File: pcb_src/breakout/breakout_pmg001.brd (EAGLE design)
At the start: 25.4 x 60.3 mm, 26 parts

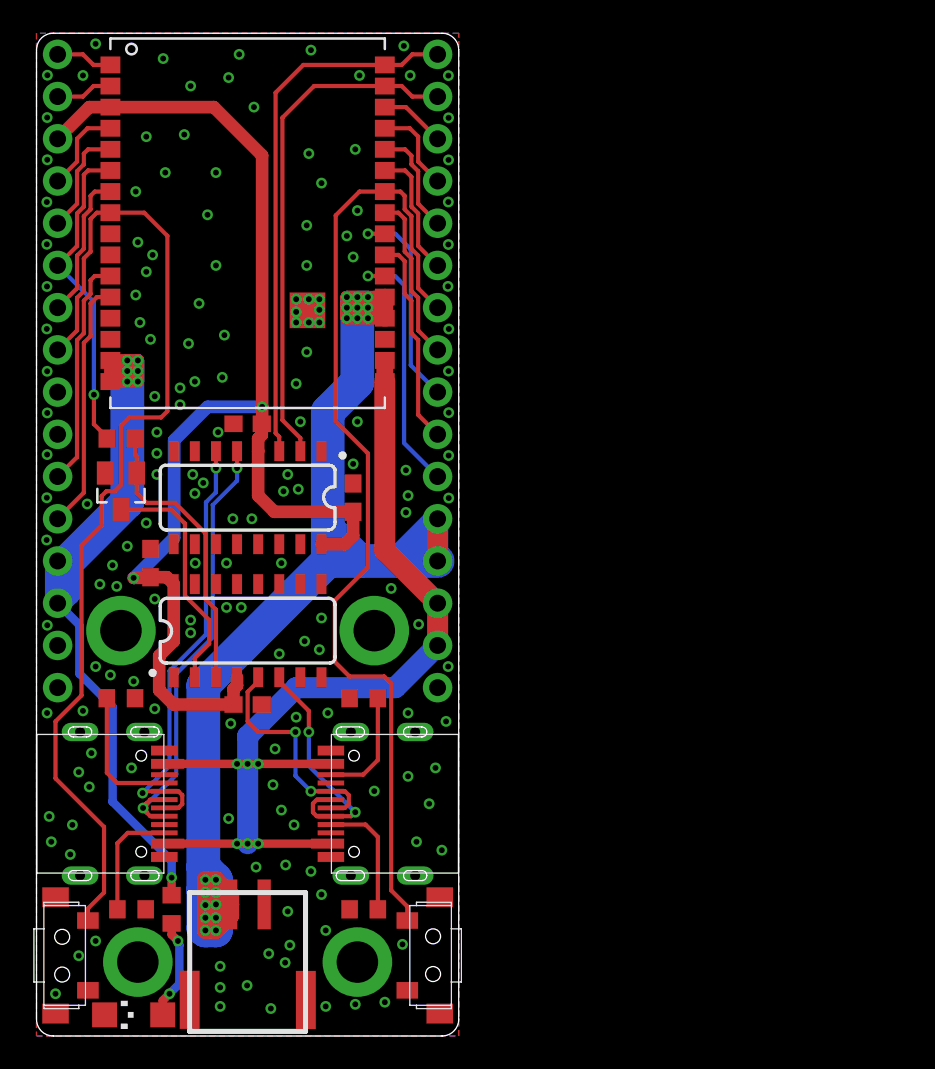
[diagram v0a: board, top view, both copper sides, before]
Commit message: Reworked repository
Name changed, added a lot of new resources etc.
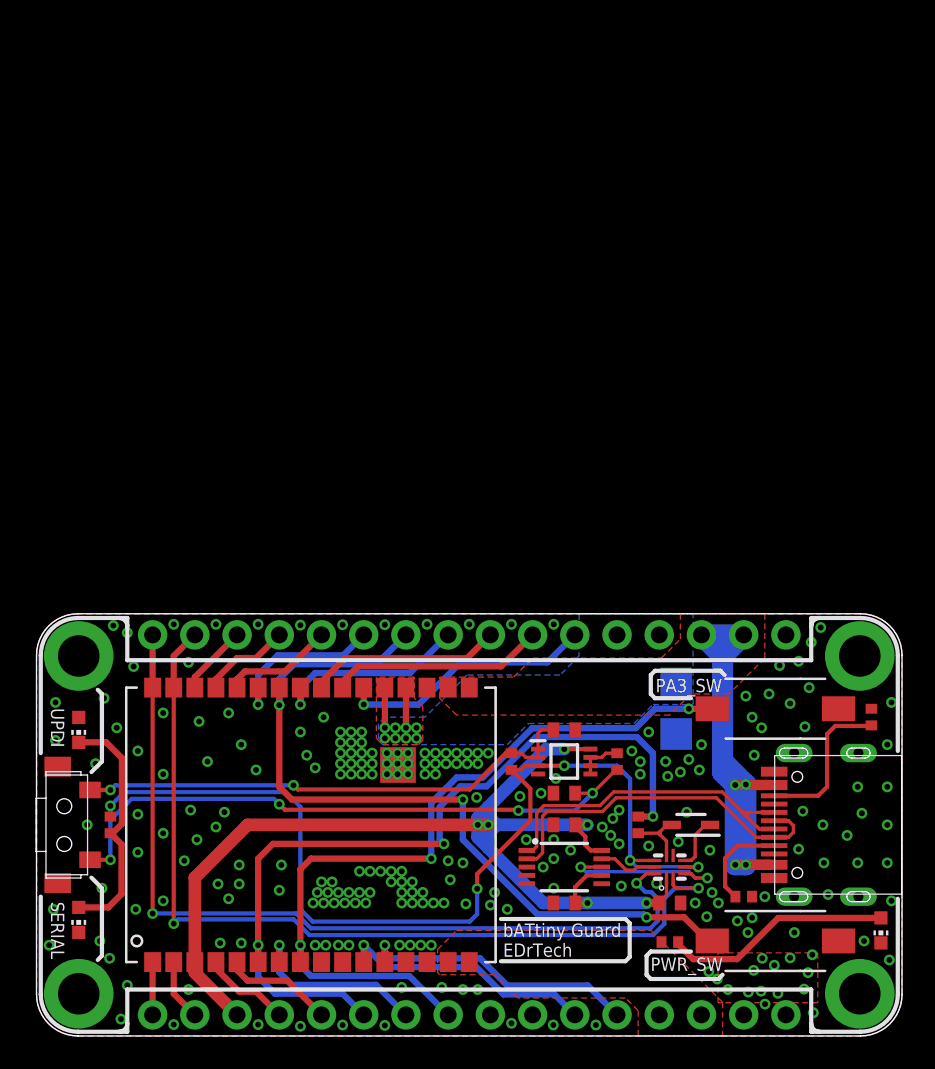
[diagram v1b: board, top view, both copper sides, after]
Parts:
- removed C3, C4, C5, C6: 100nF, eagle-ltspice:C0603
- removed LED1: (no value), led:CHIPLED_1206
- removed R11, R12, R7: 5.1k, rcl:R0603
- removed R8: 470R, rcl:R0603
- removed SPEAKER_CON1: JST_HEADER_2MM_2P, edrtech_lib:JST_HEADER
- removed U$3: TS-1101VS-C-A-A, circuitmess_device_library:TS-1101VS-C-A-A
- removed U$5: CH340C, circuitmess_device_library:CH340C
- removed U$6: USB-C, edrtech_lib:USB-C
- added C1: 1u, rcl:C0402
- added C2: 10n, rcl:C0402
- added C7, C8, C9: 100nF, rcl:C0402
- added IC1: SN74AUP2G00DCUR, SN74AUP2G00DCUR:SOP50P310X90-8N
- added LED2, LED4, LED5: (no value), led:CHIP-LED0603
- added R1: 100k, rcl:R0402
- added R2: 10k, rcl:R0402
- added R3, R4: 5.1k, rcl:R0402
- added R9: 470R, rcl:R0402
- added S5: TS3A5223RSWR, TS3A5223RSWR:RSW(RPUQFNN10)
- added TP1, TP2: TPSQTP19SQ, testpad:TP19SQ
- added U$12: USB-C, edrtech_lib:USB-C
- added U2: CH340E_MSOP10, CH340E:MSOP10
- D1: value BAT54 -> BAT54WS-13P; device diode:SOT23 -> BAT54WS-13P:SOD2512X115N
- R5, R6: device rcl:R0603 -> rcl:R0402
- U$1: value CH340C -> TS-1101S; device circuitmess_device_library:CH340C -> edrtech_lib:TS-1101S
- U$4: value USB-C -> TS-1101S; device edrtech_lib:USB-C -> edrtech_lib:TS-1101S
- moved U$9 47.2 mm to (49.5, 22.9), turned to 90 degrees
- moved JP1 46.0 mm to (26.0, 1.27), turned to 0 degrees
- moved U$4 41.5 mm to (44.5, 5.71), turned to 180 degrees
- moved D1 39.7 mm to (39.4, 12.7)
- moved U$7 36.4 mm to (16.5, 12.7), turned to 90 degrees
- moved U$1 34.2 mm to (44.5, 19.7)
- moved U$8 30.3 mm to (49.5, 2.54), turned to 90 degrees
- moved R5 30.0 mm to (38.1, 5.65), turned to 180 degrees
- moved U$10 22.0 mm to (2.54, 2.54), turned to 90 degrees
- moved U$11 17.8 mm to (2.54, 22.9), turned to 90 degrees
- moved R6 16.1 mm to (4.45, 12.7), turned to 90 degrees
- moved JP2 16.0 mm to (26.0, 24.1), turned to 180 degrees
- moved U$2 7.86 mm to (1.27, 12.7)
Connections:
- removed net D+_AT: U$1.5, U$4.DP1, U$4.DP2
- removed net D+_U: U$5.5, U$6.DP1, U$6.DP2
- removed net D-_AT: U$1.6, U$4.DN1, U$4.DN2
- removed net D-_U: U$5.6, U$6.DN1, U$6.DN2
- removed net N$5: R7.1, U$6.CC2
- removed net N$8: R11.2, U$4.CC1
- removed net N$9: R12.1, U$4.CC2
- new net D+: U$12.DP1, U$12.DP2, U2.1
- new net D-: U$12.DN1, U$12.DN2, U2.2
- new net N$1: C2.2, IC1.1, IC1.2, R2.1, U$2.P$4
- new net N$11: C1.1, R1.1, U$2.P$3
- new net N$2: R3.2, U$12.CC1
- new net N$6: R4.1, U$12.CC2
- new net N$7: IC1.5, IC1.6, IC1.7, R1.2
- new net RXI: S5.9, U2.9
- new net SEL: IC1.3, R2.2, R6.2, S5.4, S5.8
- new net TXO: S5.3, U2.8
- net 3V3: now also C7.2, C8.2, C9.1, IC1.8, S5.1, U2.10, U2.7; no longer C3.2, C4.2, C5.2, C6.2, U$1.16, U$1.4, U$5.16, U$5.4
- net 5V: now also U$12.VCC@1, U$12.VCC@2; no longer U$4.VCC@1, U$4.VCC@2, U$6.VCC@1, U$6.VCC@2
- net AT_RXD: now also S5.2; no longer U$1.2
- net AT_TXD: now also S5.10; no longer U$1.3
- net BAT: now also TP1.TP; no longer SPEAKER_CON1.+
- net GND: now also C1.2, C2.1, C7.1, C8.1, C9.2, IC1.4, LED2.C, LED4.A, LED5.C, R3.1, R4.2, S5.6, TP2.TP, U$1.P$1, U$12.GND@1, U$12.GND@2, U$12.P$1, U$12.P$2, U$12.P$3, U$12.P$4, U2.3; no longer C3.1, C4.1, C5.1, C6.1, LED1.C, R11.1, R12.2, R6.1, R7.2, SPEAKER_CON1.-, U$1.1, U$2.P$3, U$3.P$4, U$4.GND@1, U$4.GND@2, U$4.P$2, U$4.P$3, U$4.P$4, U$5.1, U$6.GND@1, U$6.GND@2, U$6.P$1, U$6.P$2, U$6.P$3, U$6.P$4
- net N$3: now also LED2.A; no longer LED1.A
- net N$4: now also LED4.C, LED5.A, R6.1; no longer R6.2, U$6.CC1
- net PA3: now also U$1.P$2; no longer U$2.P$4
- net PWR_SW: now also U$4.P$2; no longer U$3.P$3
- net UPDI: now also R9.1; no longer R8.1
- net UPDI_RX: now also D1.2, R9.2, S5.7; no longer D1.1, R8.2, U$5.3
- net UPDI_TX: now also D1.1, S5.5; no longer D1.3, U$5.2
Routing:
- net BAT: track 104.7 -> 4.83 mm, vias 19 -> 8
- net SEL: track 0.00 -> 59.6 mm, vias 0 -> 5
- net BAT_OUT: track 53.0 -> 0.00 mm, vias 7 -> 0
- net N$11: track 0.00 -> 37.0 mm, vias 0 -> 4
- net N$1: track 0.00 -> 30.6 mm, vias 0 -> 2
- net UPDI: track 19.5 -> 49.0 mm, vias 1 -> 3
- net 5V: track 60.4 -> 31.4 mm, vias 6 -> 4
- net D+_AT: track 27.4 -> 0.00 mm, vias 2 -> 0
- net D-_AT: track 26.6 -> 0.00 mm, vias 2 -> 0
- net AT_RXD: track 30.9 -> 54.0 mm, vias 0 -> 2
- net D-: track 0.00 -> 21.6 mm
- net D+: track 0.00 -> 20.6 mm
- net AT_TXD: track 32.4 -> 52.0 mm, vias 0 -> 2
- net D-_U: track 14.5 -> 0.00 mm, vias 2 -> 0
- net D+_U: track 14.1 -> 0.00 mm, vias 2 -> 0
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- added copper zone on layer 1, net 5V
- added copper zone on layer 1, net BAT
- added copper zone on layer 16, net BAT
- added copper zone on layer 1, net BAT_OUT
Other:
- board size 25.4 x 60.3 mm -> 52.1 x 25.4 mm
- board text added: "BAT OUT"
- board text added: "BAT+"
- board text added: "BAT-"
- board text added: "PA3_SW"
- board text added: "PA7"
- board text added: "PB0"
- board text added: "PB1"
- board text added: "bATtiny Guard"
- board text added: "bATtiny Guard EDrTech"
- board text removed: "BAT"
- board text removed: "BATTERY"
- board text removed: "CLK"
- board text removed: "PA3 SW"
- board text removed: "PMG001 Breakout board"
- board text removed: "SDA"
